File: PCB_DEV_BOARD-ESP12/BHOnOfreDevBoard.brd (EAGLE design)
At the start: 53 x 55 mm, 25 parts, among them K1 OMRON-G3MB-202P-SSR2, K2 OMRON-G3MB-202P-SSR2, Q1 S8050, Q2 S8050, SW1 B3U-1000P-2P-SMD

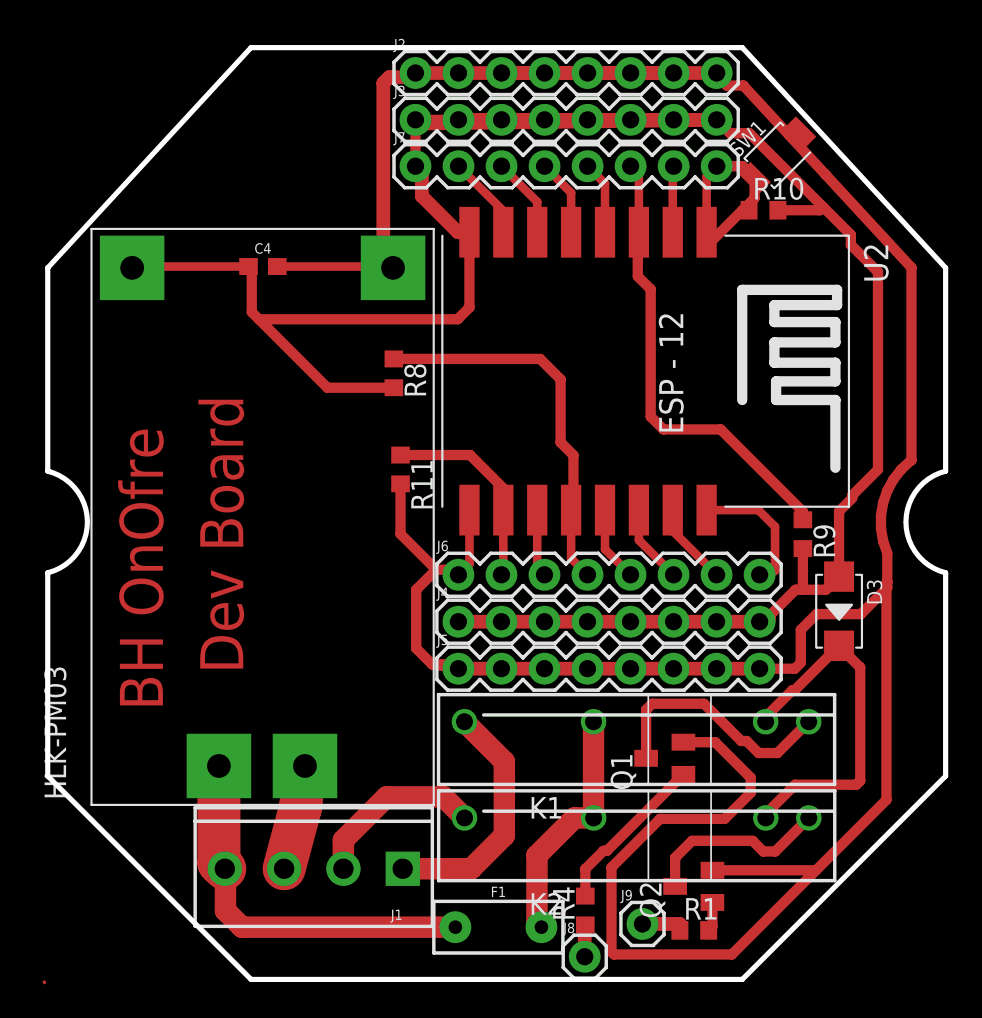
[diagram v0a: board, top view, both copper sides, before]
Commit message: ficheiros para fazer a PCB na CNC
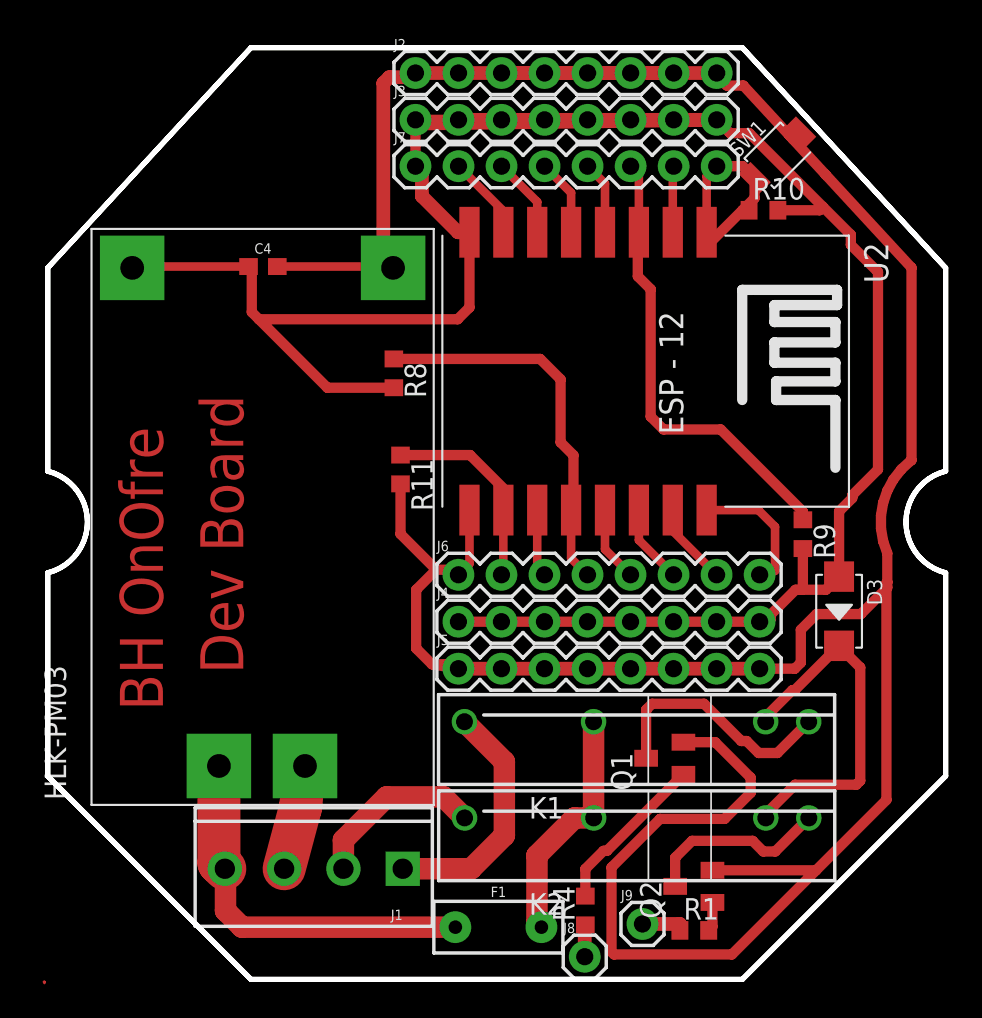
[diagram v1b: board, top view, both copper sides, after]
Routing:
- net VCC: track 175.9 -> 158.1 mm
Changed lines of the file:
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@@
 <layer number="23" name="tOrigins" color="15" fill="1" visible="yes" active="yes"/>
 <layer number="24" name="bOrigins" color="15" fill="1" visible="yes" active="yes"/>
-<layer number="25" name="tNames" color="7" fill="1" visible="no" active="yes"/>
-<layer number="26" name="bNames" color="7" fill="1" visible="no" active="yes"/>
-<layer number="27" name="tValues" color="7" fill="1" visible="no" active="yes"/>
+<layer number="25" name="tNames" color="7" fill="1" visible="yes" active="yes"/>
+<layer number="26" name="bNames" color="7" fill="1" visible="yes" active="yes"/>
+<layer number="27" name="tValues" color="7" fill="1" visible="yes" active="yes"/>
 <layer number="28" name="bValues" color="7" fill="1" visible="yes" active="yes"/>
 <layer number="29" name="tStop" color="7" fill="3" visible="no" active="yes"/>
@@
 <text x="6.99344375" y="16.011896875" size="2.54" layer="1" font="vector" rot="R90">BH OnOfre</text>
 <text x="11.73625625" y="18.18410625" size="2.54" layer="1" font="vector" rot="R90">Dev Board</text>
+<wire x1="53.19408125" y1="12.145271875" x2="41.19408125" y2="0.145271875" width="0.3048" layer="46"/>
+<wire x1="41.19408125" y1="0.145271875" x2="12.19408125" y2="0.145271875" width="0.3048" layer="46"/>
+<wire x1="12.19408125" y1="0.145271875" x2="0.19408125" y2="12.145271875" width="0.3048" layer="46"/>
+<wire x1="0.19408125" y1="12.145271875" x2="0.19408125" y2="24.145271875" width="0.3048" layer="46"/>
+<wire x1="0.19408125" y1="30.145271875" x2="0.19408125" y2="42.145271875" width="0.3048" layer="46"/>
+<wire x1="0.19408125" y1="42.145271875" x2="12.19408125" y2="55.145271875" width="0.3048" layer="46"/>
+<wire x1="12.19408125" y1="55.145271875" x2="41.19408125" y2="55.145271875" width="0.3048" layer="46"/>
+<wire x1="41.19408125" y1="55.145271875" x2="53.19408125" y2="42.145271875" width="0.3048" layer="46"/>
+<wire x1="53.19408125" y1="42.145271875" x2="53.19408125" y2="30.145271875" width="0.3048" layer="46"/>
+<wire x1="53.19408125" y1="24.145271875" x2="53.19408125" y2="12.145271875" width="0.3048" layer="46"/>
+<wire x1="53.19408125" y1="24.145271875" x2="53.19408125" y2="30.145271875" width="0.3048" layer="46" curve="-151.927513"/>
+<wire x1="0.19408125" y1="30.145271875" x2="0.19408125" y2="24.145271875" width="0.3048" layer="46" curve="-151.927513"/>
 </plain>
 <attributes>
@@
 <wire x1="34.60115" y1="50.88254375" x2="36.8927625" y2="50.88254375" width="0.6096" layer="1"/>
 <wire x1="37.14115" y1="50.88254375" x2="39.68115" y2="50.88254375" width="0.6096" layer="1"/>
-<wire x1="42.215521875" y1="21.25885" x2="24.435521875" y2="21.25885" width="0.8128" layer="1"/>
 </signal>
 <signal name="N$1">
